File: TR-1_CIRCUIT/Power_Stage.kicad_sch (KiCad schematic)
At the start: 7 parts, among them SW1 SW_SPDT, U2 AZ1084-1.2

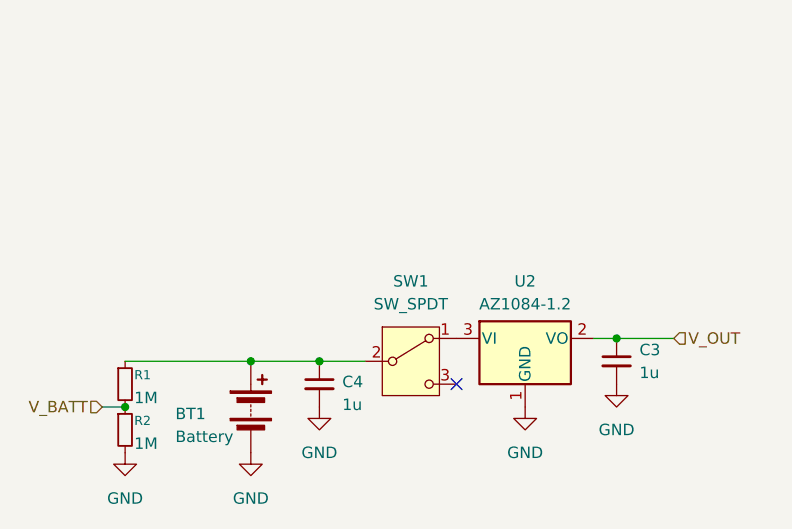
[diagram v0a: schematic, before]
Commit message: Finalized circuit design + README
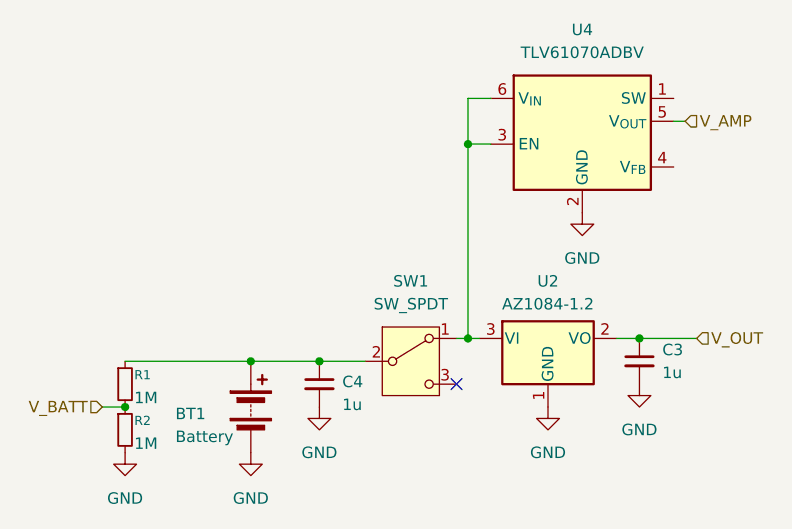
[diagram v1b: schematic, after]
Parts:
- added U4: TLV61070ADBV, Package_TO_SOT_SMD:SOT-23-6, symbol Regulator_Switching:TLV61070ADBV
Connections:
- net GND: now also U4.2 (GND)
- net at SW1.1 (A), U2.3 (VI): now also U4.3 (EN), U4.6 (V_{IN})
- new net V_AMP: U4.5 (V_{OUT})
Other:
- moved on the sheet: C3, U2
